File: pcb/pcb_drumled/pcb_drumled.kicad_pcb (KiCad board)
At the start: 2 copper layers, 46.4 x 28.6 mm, 20 parts, among them J1 Conn_02x07_Odd_Even, U1 STM32G431KBTx

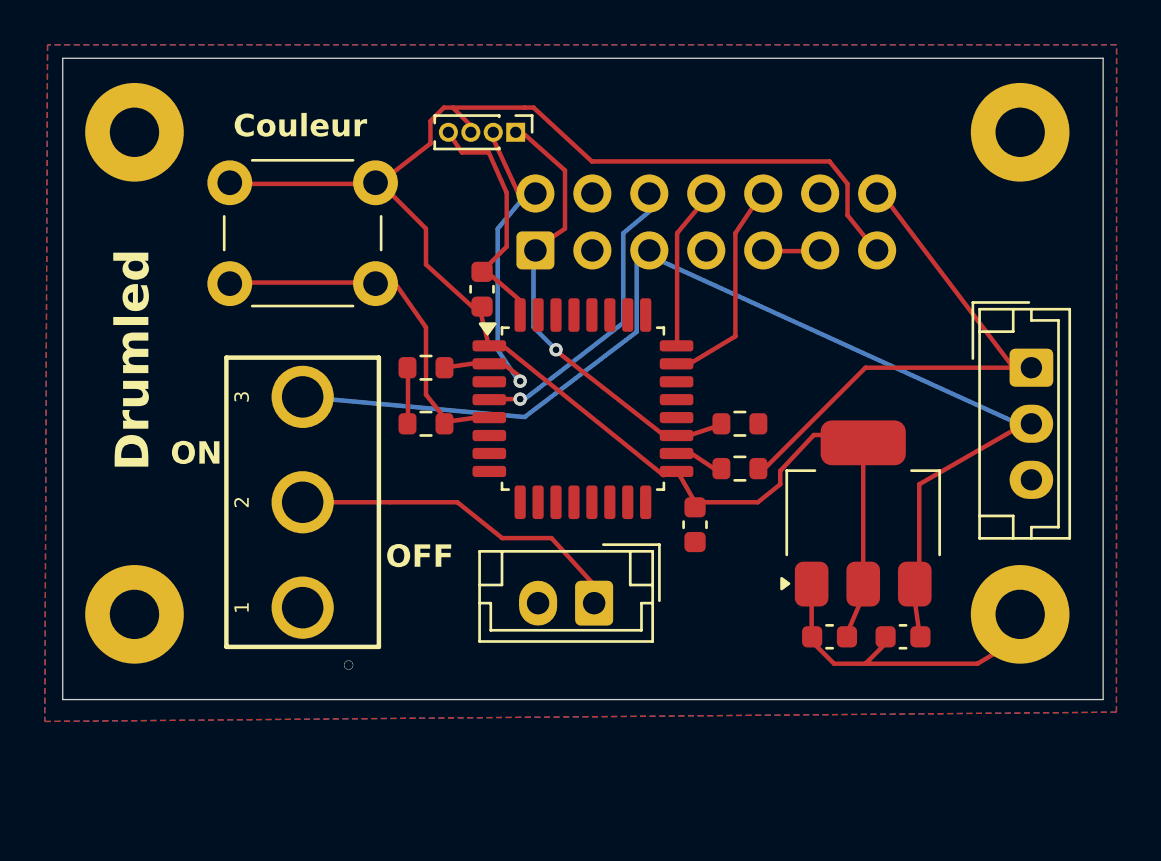
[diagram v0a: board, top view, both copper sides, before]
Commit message: pcb_fini
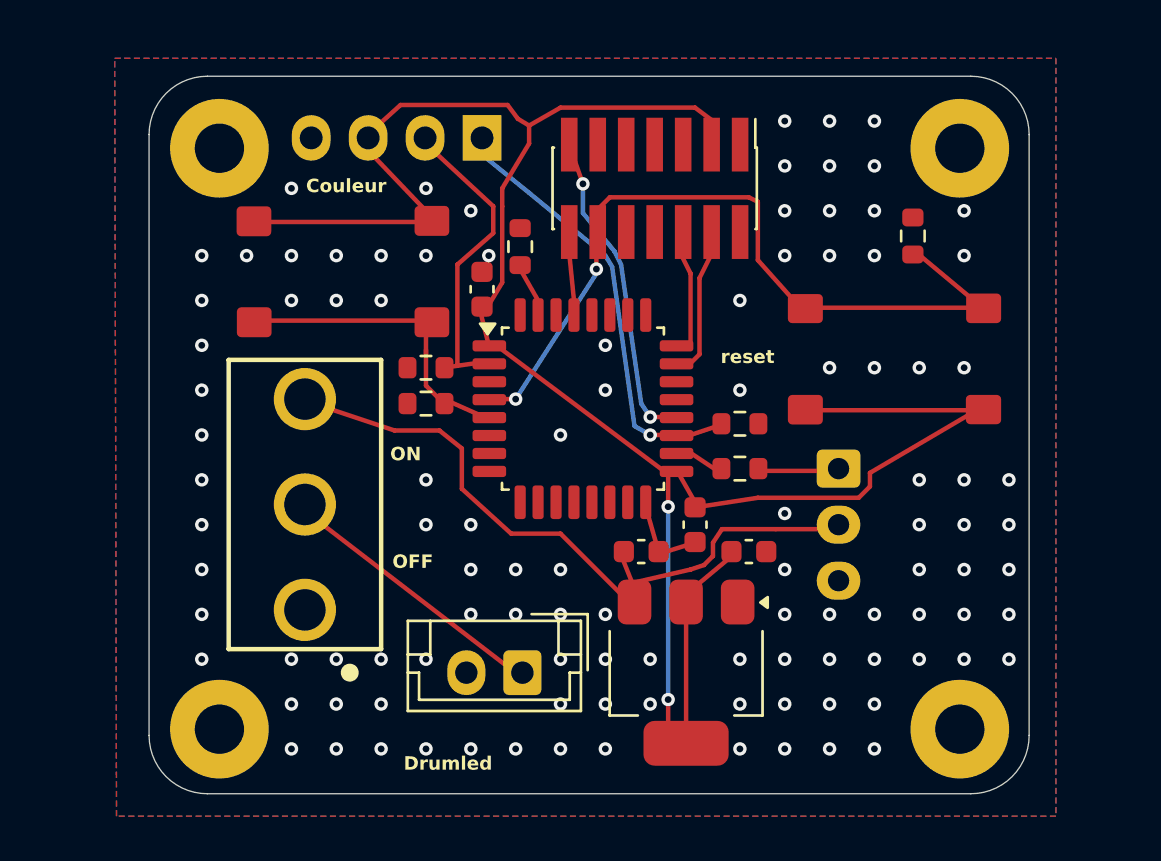
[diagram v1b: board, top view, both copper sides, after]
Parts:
- removed J1: Conn_02x07_Odd_Even, Connector_IDC:IDC-Header_2x07_P2.54mm_Vertical
- added J2: Conn_ST_STDC14, Connector_PinHeader_1.27mm:PinHeader_2x07_P1.27mm_Vertical_SMD, F.Cu at (228.2, 47.0)
- added R3: 10k, Resistor_SMD:R_0603_1608Metric, F.Cu at (239.7, 49.1)
- added R5: 10k, Resistor_SMD:R_0603_1608Metric, F.Cu at (222.2, 49.6)
- added reset1: SW_Push, Library:button, F.Cu at (239.7, 49.1)
- bouton_couleur1: footprint Button_Switch_THT:SW_PUSH_6mm -> Library:button
- connecteur_capteur1: footprint Connector_PinHeader_1.00mm:PinHeader_1x04_P1.00mm_Vertical -> Connector:FanPinHeader_1x04_P2.54mm_Vertical
- rgb_neopix1: footprint Connector_JST:JST_EH_B3B-EH-A_1x03_P2.50mm_Vertical -> Connector_JST:JST_EH_S3B-EH_1x03_P2.50mm_Horizontal
- moved C1 12.3 mm to (227.6, 63.2), turned to 180 degrees
- moved regulateur_vers_3.3V1 10.6 mm to (229.6, 68.6), turned to -90 degrees
- moved rgb_neopix1 9.71 mm to (236.4, 59.5)
- moved H2 6.37 mm to (208.8, 71.1)
- moved bouton_couleur1 6.06 mm to (215.1, 45.2), turned to 0 degrees
- moved H5 5.78 mm to (241.8, 71.1)
- moved C4 5.23 mm to (232.4, 63.2), turned to 180 degrees
- moved connecteur_batterie1 4.46 mm to (222.3, 68.6)
- moved H1 3.85 mm to (208.8, 45.2)
- moved H3 2.78 mm to (241.8, 45.2)
- moved connecteur_capteur1 1.52 mm to (220.5, 44.8), turned to 180 degrees
- moved R4 0.90 mm to (218.0, 56.6)
- moved switch_on_off1 0.14 mm to (212.6, 61.1)
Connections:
- C1 pad 1: 0 -> GND
- C2 pad 2: 0 -> GND
- C3 pad 1: 0 -> GND
- C4 pad 1: 0 -> GND
- H1 pad 1: 0 -> GND
- H2 pad 1: 0 -> GND
- H3 pad 1: 0 -> GND
- H5 pad 1: 0 -> GND
- R1 pad 2: 0 -> GND
- R2 pad 2: 0 -> GND
- R4 pad 2: 0 -> GND
- U1 pad 14: 0 -> GND
- U1 pad 15: 0 -> GND
- U1 pad 16: 0 -> GND
- U1 pad 20: unconnected-(U1-PA10-Pad20) -> RX
- U1 pad 29: unconnected-(U1-PB6-Pad29) -> TX
- U1 pad 31: unconnected-(U1-PB8-Pad31) -> Net-(U1-PB8)
- U1 pad 32: 0 -> GND
- bouton_couleur1 pad 1: PA0 -> 3.3V
- bouton_couleur1 pad 2: 3.3V -> PA0
- connecteur_batterie1 pad 2: 0 -> GND
- connecteur_capteur1 pad 4: 0 -> GND
- regulateur_vers_3.3V1 pad 1: 0 -> GND
- rgb_neopix1 pad 3: 0 -> GND
- switch_on_off1 pad 1: 0 -> unconnected-(switch_on_off1-C-Pad1)
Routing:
- net SDA: vias 1 -> 0
- net RX: vias 0 -> 2
- net RESET: vias 1 -> 2
- net GND: vias 0 -> 102
- net 3.3V: vias 0 -> 2
- net (no net): vias 0 -> 6
- added copper zone on B.Cu, net GND
- added copper zone on F.Cu, net GND
- removed copper zone on B.Cu, net 0
- removed copper zone on F.Cu, net 0
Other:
- board size 46.4 x 28.6 mm -> 39.3 x 32 mm
- board text added: "reset"
